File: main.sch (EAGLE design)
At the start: 14 parts, among them IC1 ATMEGA328P-PU, IC2 LM7805, J1 2,1mm, Q1 16 MHz

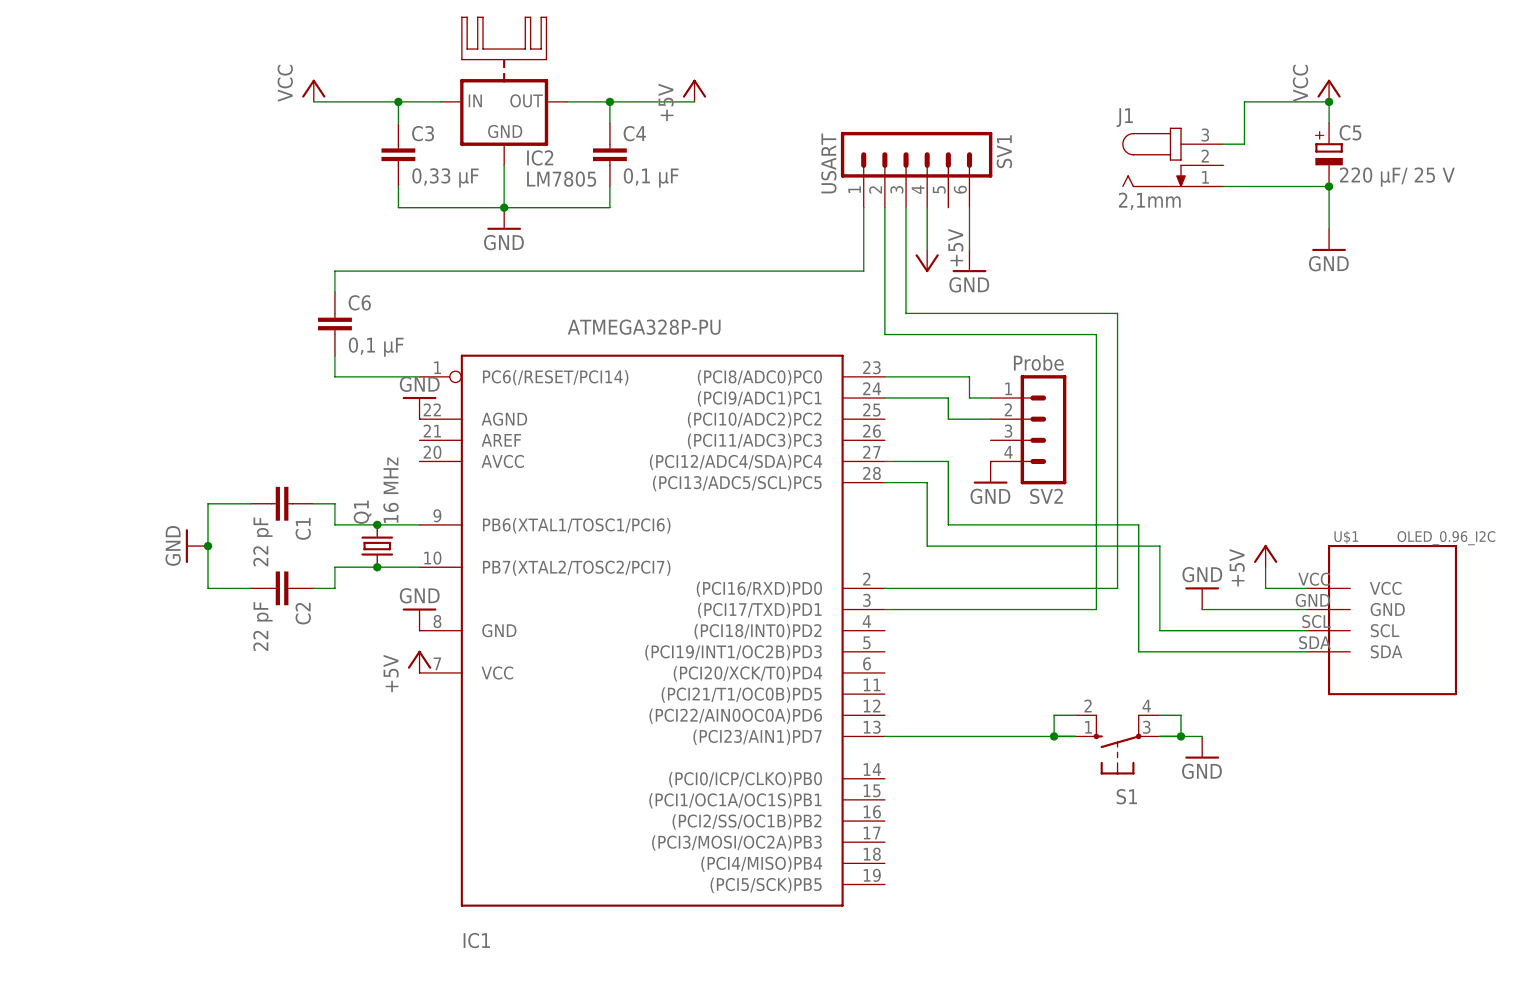
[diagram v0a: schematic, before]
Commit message: Minor fixes
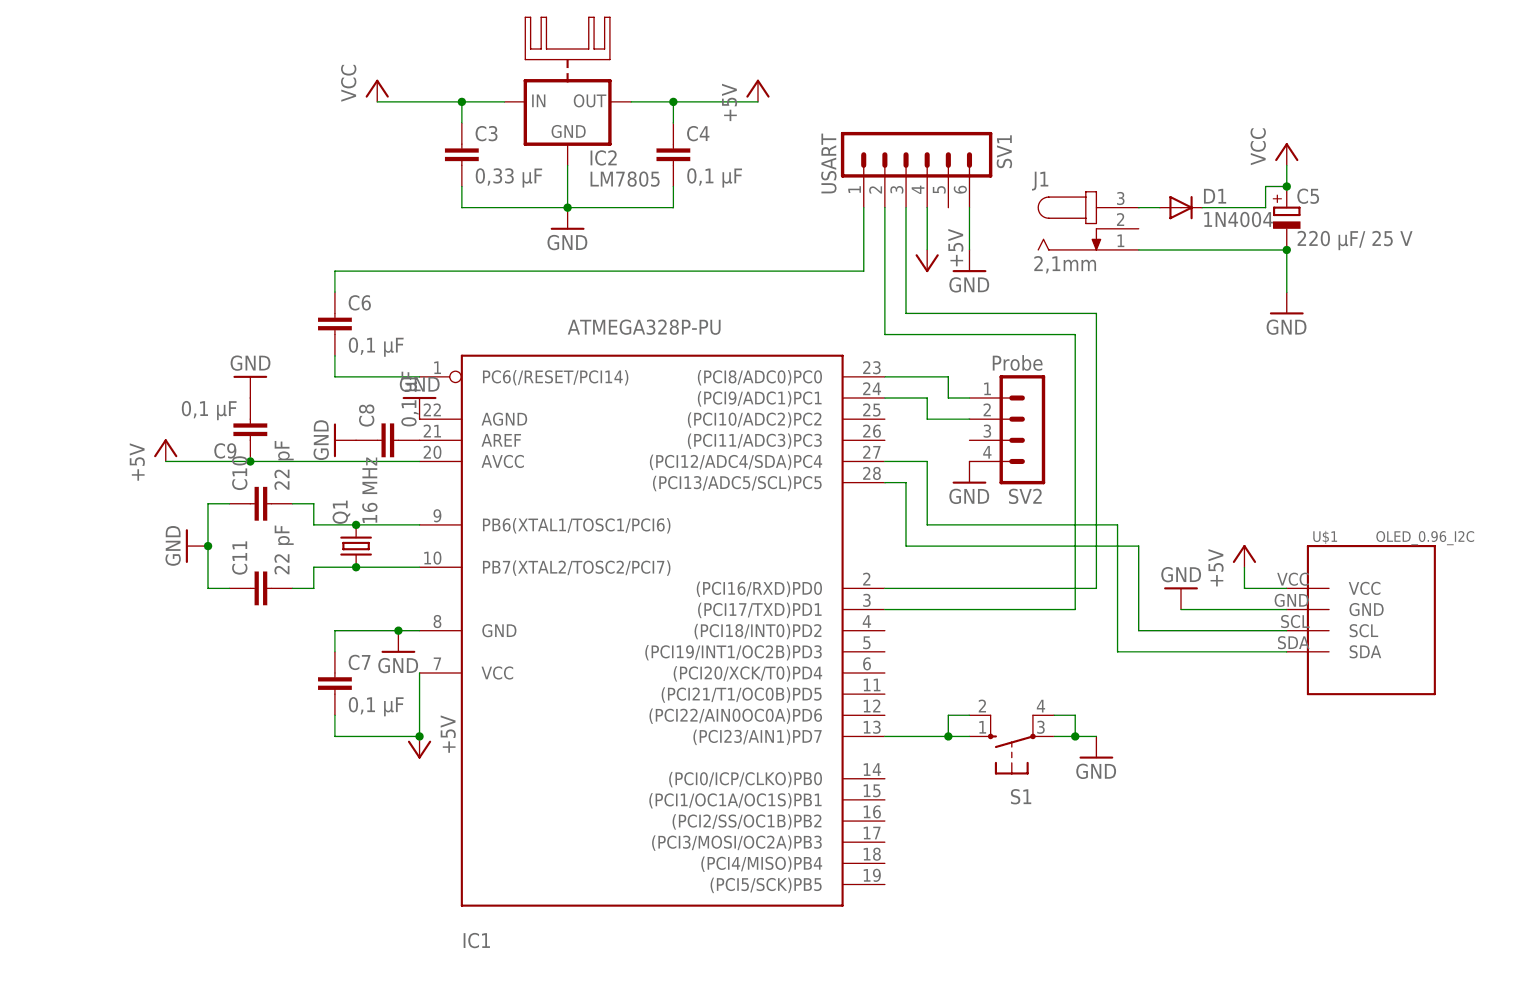
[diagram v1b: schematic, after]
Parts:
- removed C1, C2: 22 pF, capacitor-wima:C2.5/2
- added C10, C11: 22 pF, rcl:C-EU025-025X050
- added C7, C8, C9: 0,1 μF, rcl:C-EU050-025X075
- added D1: 1N4004, diode:1N4004
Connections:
- new net N$12: C8.2, IC1.AREF
- new net N$13: D1.A, J1.3
- net +5V: now also C7.2, C9.1, IC1.AVCC
- net GND: now also C10.1, C11.1, C7.1, C8.1, C9.2; no longer C1.2, C2.2
- net N$1: now also C11.2; no longer C2.1
- net N$2: now also C10.2; no longer C1.1
- net VCC: now also D1.C; no longer J1.3
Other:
- moved on the sheet: C3, C4, C5, IC2, J1, Q1, S1, SV2, U$1

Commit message: Opravy
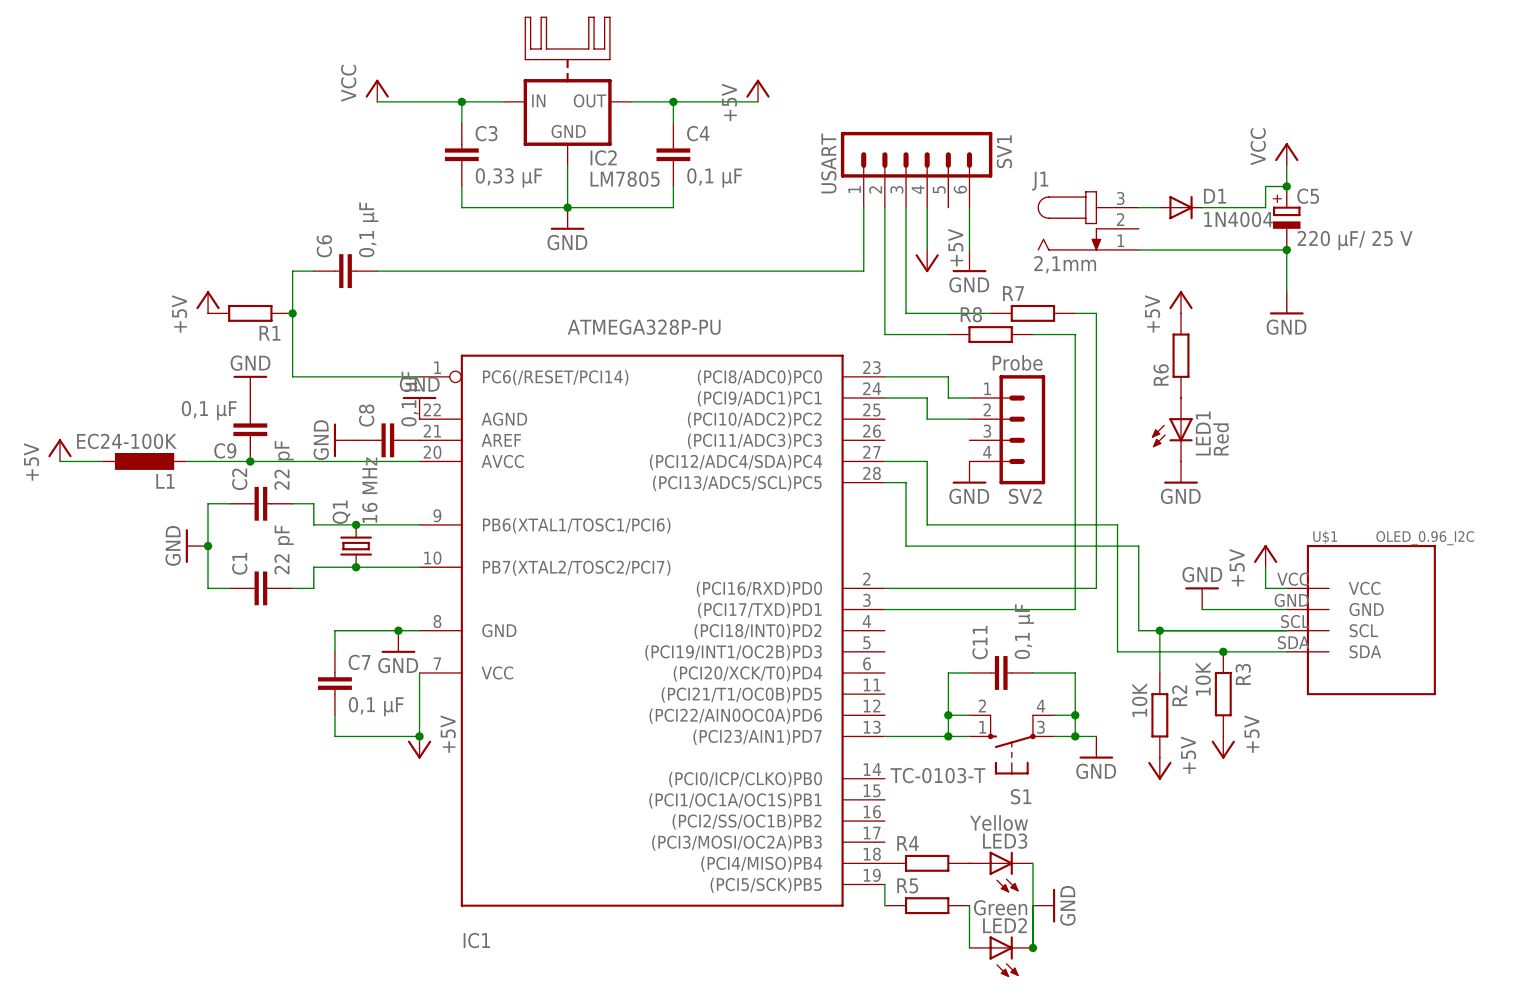
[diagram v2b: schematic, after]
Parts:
- added C1: 22 pF, rcl:C-EU025-025X050
- added L1: EC24-100K, rcl:L-EU0207/12
- added LED1: Red, led:LED5MM
- added LED2: Green, led:LED5MM
- added LED3: Yellow, led:LED5MM
- added R1, R4, R5, R6, R7, R8: (no value), rcl:R-EU_0207/7
- added R2, R3: 10K, rcl:R-EU_0207/7
- C11: value 22 pF -> 0,1 μF; device rcl:C-EU025-025X050 -> rcl:C-EU050-025X075
- S1: value (none) -> TC-0103-T
- renumbered C10 to C2
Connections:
- new net N$14: IC1.(PCI4/MISO)PB4, R4.1
- new net N$16: IC1.(PCI5/SCK)PB5, R5.1
- new net N$17: LED3.A, R4.2
- new net N$18: C9.1, IC1.AVCC, L1.2
- new net N$19: LED2.A, R5.2
- new net N$20: LED1.A, R6.1
- new net N$21: R8.1, SV1.2
- new net N$22: R7.1, SV1.3
- net +5V: now also L1.1, R1.2, R2.2, R3.2, R6.2; no longer C9.1, IC1.AVCC
- net GND: now also C1.1, C11.2, LED1.C, LED2.C, LED3.C; no longer C11.1
- net N$1: now also C1.2; no longer C11.2
- net N$3: now also R3.1
- net N$4: now also R2.1
- net N$5: now also C6.1, R1.1; no longer C6.2
- net N$6: now also C11.1
- net N$7: now also C6.2; no longer C6.1
- net N$8: now also R7.2; no longer SV1.3
- net N$9: now also R8.2; no longer SV1.2
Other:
- moved on the sheet: C11, C6
